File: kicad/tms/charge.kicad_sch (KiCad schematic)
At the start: 33 parts, among them K1 AZ9861-1C-24DC2R1, Q1 NPN, T1 Transformer_1P_1S, U1 VO2611, U2 VO2611, U7 LM393

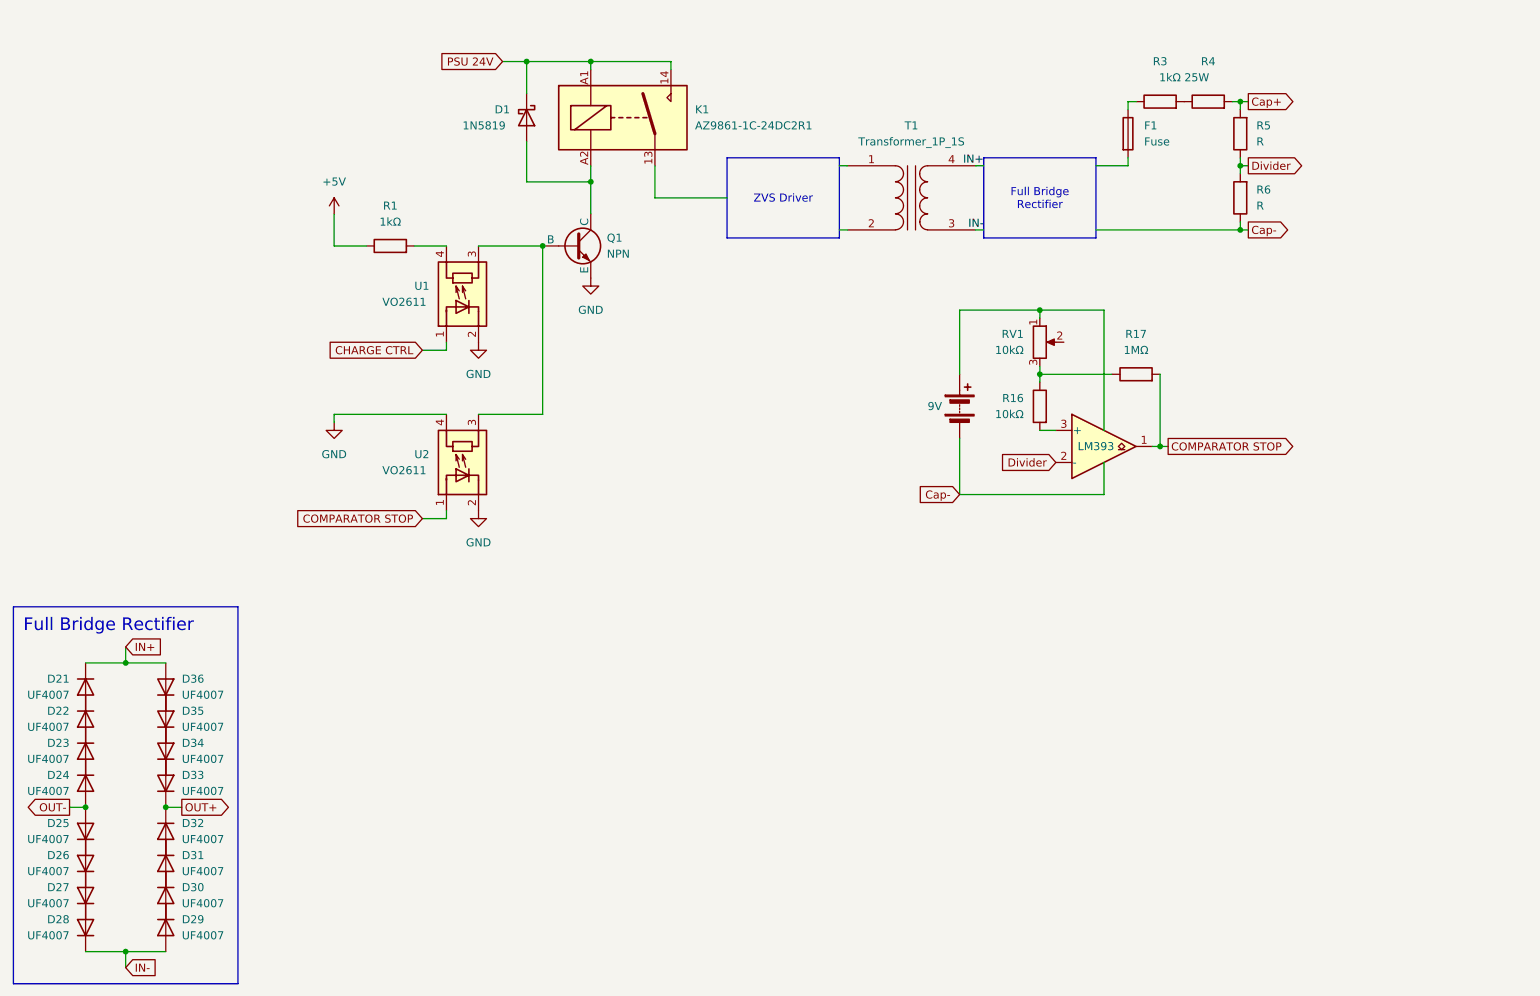
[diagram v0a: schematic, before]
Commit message: Kicad files
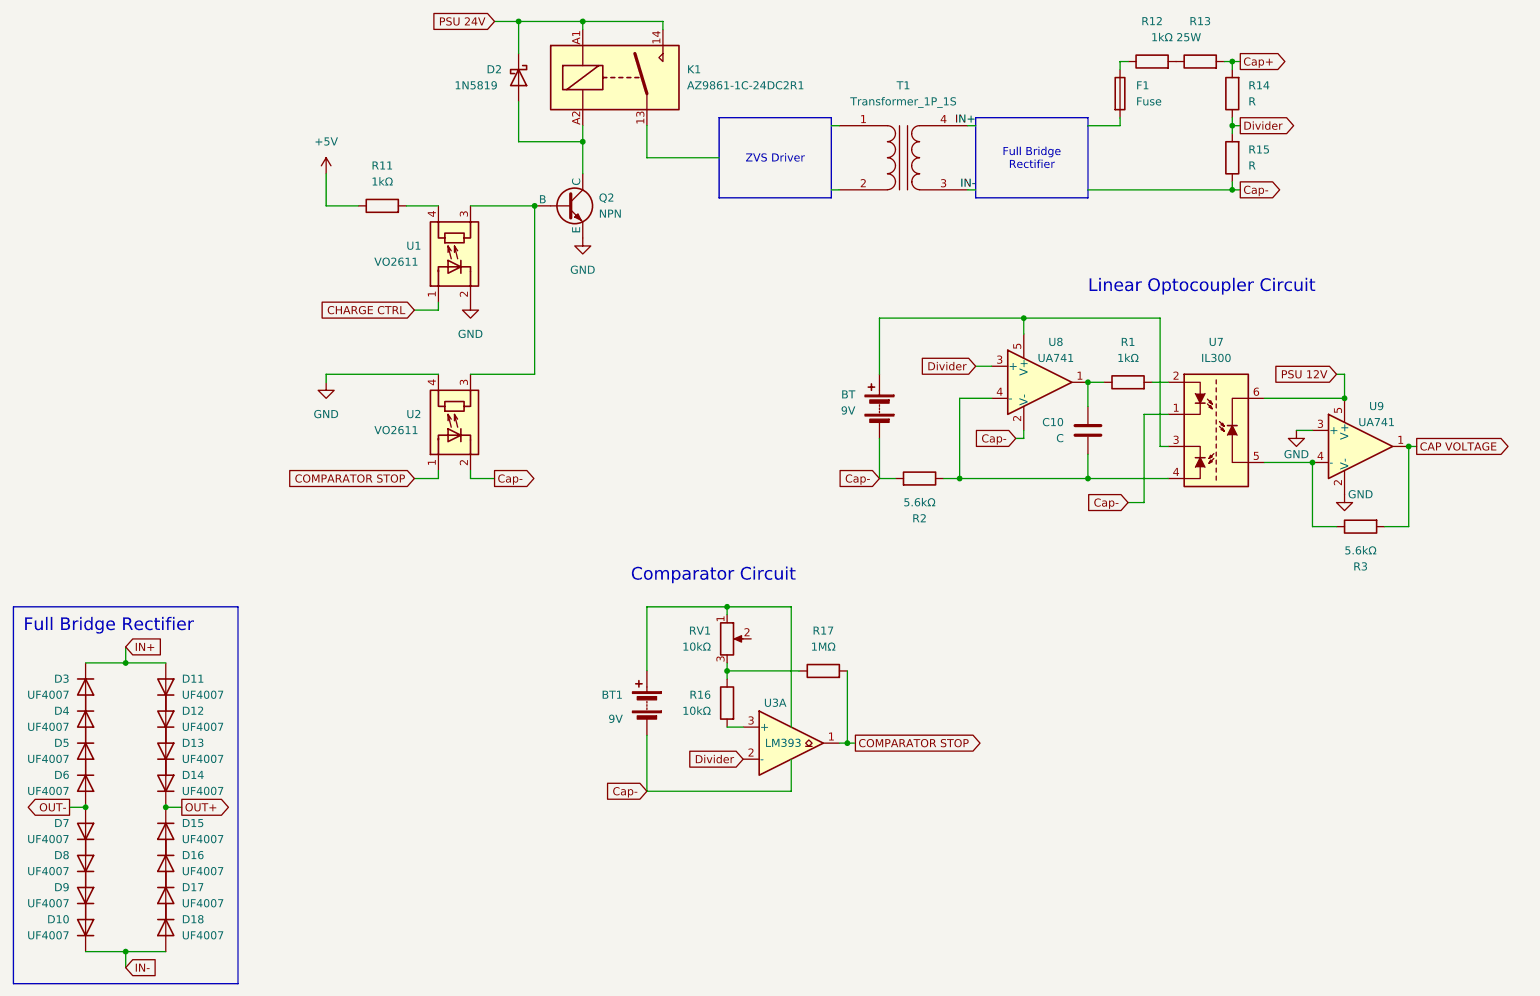
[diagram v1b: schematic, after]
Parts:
- added BT: 9V, symbol Device:Battery
- added C10: C, symbol Device:C
- added R1: 1kΩ, symbol Device:R
- added R2, R3: 5.6kΩ, symbol Device:R
- added U7: IL300, symbol Isolator_Analog:IL300
- added U8, U9: UA741, Package_TO_SOT_SMD:SOT-23-5, symbol Amplifier_Operational:ADA4610-1xRJ
- renumbered D28 to D10, D36 to D11, D35 to D12, D34 to D13, D33 to D14, D32 to D15, D31 to D16, D30 to D17, D29 to D18, D1 to D2, D21 to D3, D22 to D4, D23 to D5, D24 to D6, D25 to D7, D26 to D8, D27 to D9, Q1 to Q2, R1 to R11, R3 to R12, R4 to R13, R5 to R14, R6 to R15, U7 to U3
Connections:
- net Cap-: now also U2.2 (K), BT.2 (-), R2.2, U7.1, U8.2 (V-)
- net Divider: now also U8.3 (+)
- net GND: now also U9.2 (V-), U9.3 (+); no longer U2.2 (K)
- new net: R1.2, U7.2
- new net: BT.1 (+), U7.3, U8.5 (V+)
- new net: C10.2, R2.1, U7.4, U8.4 (-)
- new net: R3.1, U7.5, U9.4 (-)
- new net: C10.1, R1.1, U8.1
- new net CAP VOLTAGE: R3.2, U9.1
- new net PSU 12V: U7.6, U9.5 (V+)
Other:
- note added: "Comparator Circuit"
- note added: "Linear Optocoupler Circuit"
- moved on the sheet: D10, D2, D3, D4, D5, D6, D7, D8, D9, F1, K1, Q2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
